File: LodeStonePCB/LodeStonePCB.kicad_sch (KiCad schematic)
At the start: 5 parts

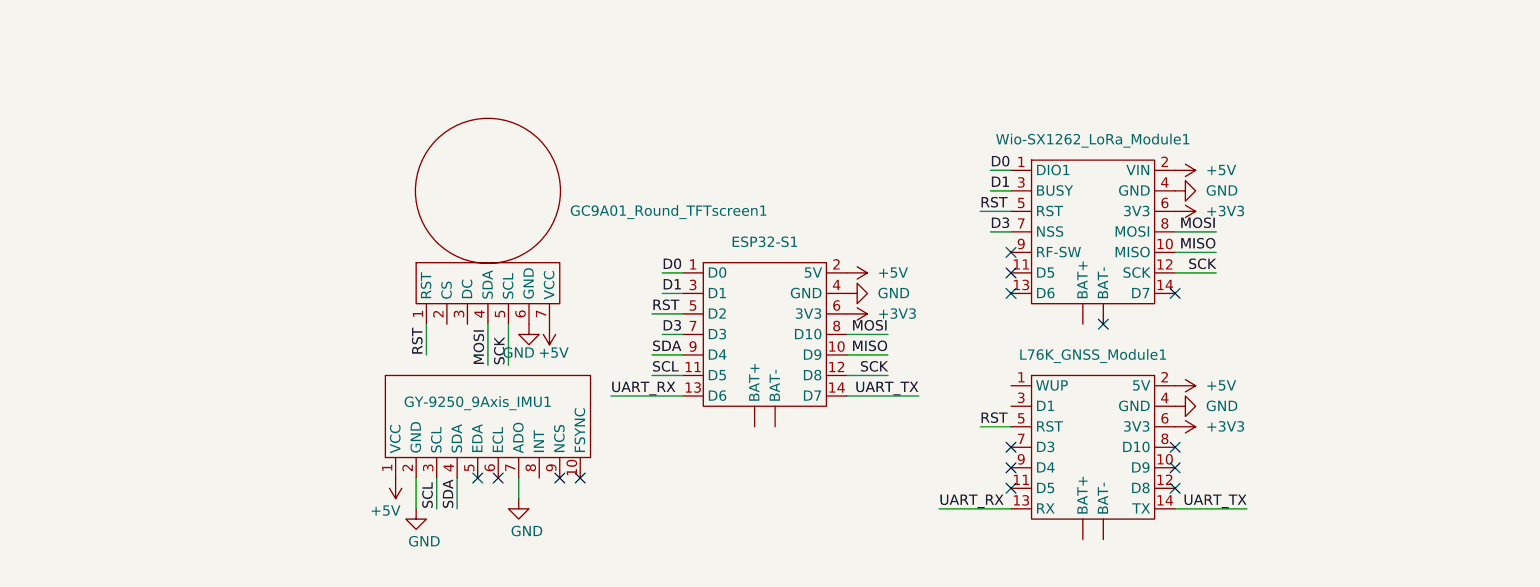
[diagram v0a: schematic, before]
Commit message: Finished pcb
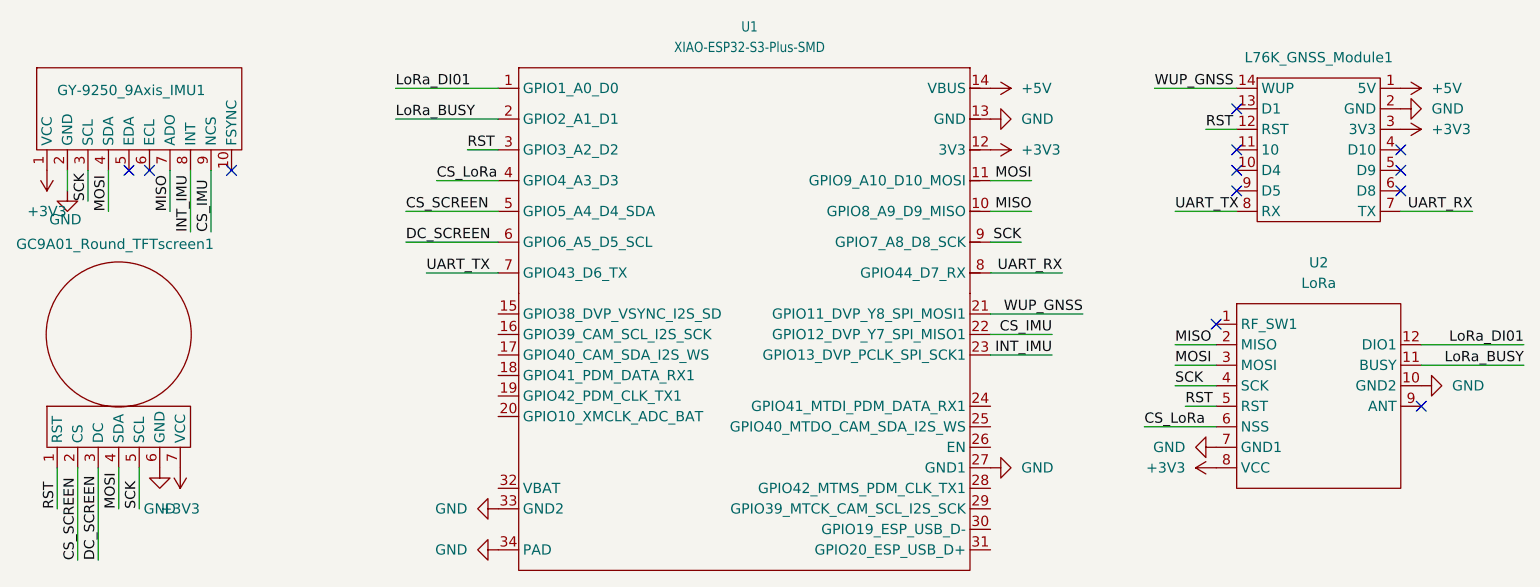
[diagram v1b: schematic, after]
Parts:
- removed ESP32-S1: (no value), symbol LodeStoneSymbols:Seeed_Studio_XIAO_ESP32_S3
- removed Wio-SX1262_LoRa_Module1: (no value), symbol LodeStoneSymbols:Wio-SX1261_Extension_Board_(LoRa)
- added U1: XIAO-ESP32-S3-Plus-SMD, LodeStoneFootprint:XIAO-ESP32-S3-Plus-SMD, symbol Seeed_Studio_XIAO_Series:XIAO-ESP32-S3 Plus-SMD
- added U2: LoRa, LodeStoneFootprint:Wio-SX1262 PCB Package, symbol LodeStoneSymbols:MODULE-WIO-SX1262
- GC9A01_Round_TFTscreen1: footprint (none) -> Connector_PinHeader_2.54mm:PinHeader_1x07_P2.54mm_Vertical
- GY-9250_9Axis_IMU1: footprint (none) -> Connector_PinHeader_2.54mm:PinHeader_1x10_P2.54mm_Vertical
- L76K_GNSS_Module1: footprint (none) -> LodeStoneFootprint:XIAO-14P-Add-On
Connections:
- net SCL is gone; now on net SCK: GY-9250_9Axis_IMU1.3 (SCL)
- net SDA is gone; now on net MOSI: GY-9250_9Axis_IMU1.4 (SDA)
- net +3V3: now also GC9A01_Round_TFTscreen1.7 (VCC), GY-9250_9Axis_IMU1.1 (VCC), L76K_GNSS_Module1.3 (3V3), U1.12 (3V3), U2.8 (VCC); no longer L76K_GNSS_Module1.6 (3V3)
- net +5V: now also L76K_GNSS_Module1.1 (5V), U1.14 (VBUS); no longer GC9A01_Round_TFTscreen1.7 (VCC), GY-9250_9Axis_IMU1.1 (VCC), L76K_GNSS_Module1.2 (5V)
- net GND: now also L76K_GNSS_Module1.2 (GND), U1.13 (GND), U1.27 (GND1), U1.33 (GND2), U1.34 (PAD), U2.10 (GND2), U2.7 (GND1); no longer GY-9250_9Axis_IMU1.7 (ADO), L76K_GNSS_Module1.4 (GND)
- net MISO: now also GY-9250_9Axis_IMU1.7 (ADO), U1.10 (GPIO8_A9_D9_MISO), U2.2 (MISO)
- net MOSI: now also U1.11 (GPIO9_A10_D10_MOSI), U2.3 (MOSI)
- net RST: now also L76K_GNSS_Module1.12 (RST), U1.3 (GPIO3_A2_D2), U2.5 (RST); no longer L76K_GNSS_Module1.5 (RST)
- net SCK: now also U1.9 (GPIO7_A8_D8_SCK), U2.4 (SCK)
- net UART_RX: now also L76K_GNSS_Module1.7 (TX), U1.8 (GPIO44_D7_RX); no longer L76K_GNSS_Module1.13 (RX)
- net UART_TX: now also L76K_GNSS_Module1.8 (RX), U1.7 (GPIO43_D6_TX); no longer L76K_GNSS_Module1.14 (TX)
- net CS_SCREEN: now reaches GC9A01_Round_TFTscreen1.2 (CS)
- net CS_SCREEN: now also U1.5 (GPIO5_A4_D4_SDA)
- net DC_SCREEN: now reaches GC9A01_Round_TFTscreen1.3 (DC)
- net DC_SCREEN: now also U1.6 (GPIO6_A5_D5_SCL)
- net INT_IMU: now reaches GY-9250_9Axis_IMU1.8 (INT)
- net INT_IMU: now also U1.23 (GPIO13_DVP_PCLK_SPI_SCK1)
- net CS_IMU: now reaches GY-9250_9Axis_IMU1.9 (NCS)
- net CS_IMU: now also U1.22 (GPIO12_DVP_Y7_SPI_MISO1)
- new net CS_LoRa: U1.4 (GPIO4_A3_D3), U2.6 (NSS)
- new net LoRa_BUSY: U1.2 (GPIO2_A1_D1), U2.11 (BUSY)
- new net LoRa_DI01: U1.1 (GPIO1_A0_D0), U2.12 (DIO1)
- new net WUP_GNSS: L76K_GNSS_Module1.14 (WUP), U1.21 (GPIO11_DVP_Y8_SPI_MOSI1)
- no-connect marks 15 -> 12
